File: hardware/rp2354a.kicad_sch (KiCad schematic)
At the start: 25 parts, among them J5 SM03B-SRSS-TB_LF__SN_, U1 RP2354A, Y1 ABM8-272-T3

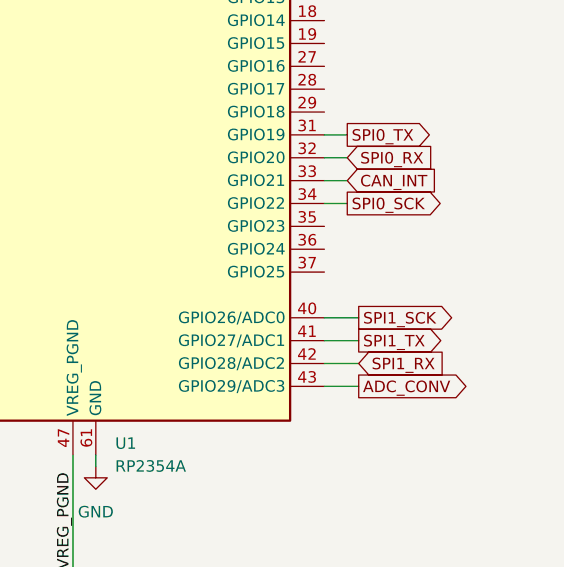
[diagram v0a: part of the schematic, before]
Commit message: Further iso bridge development
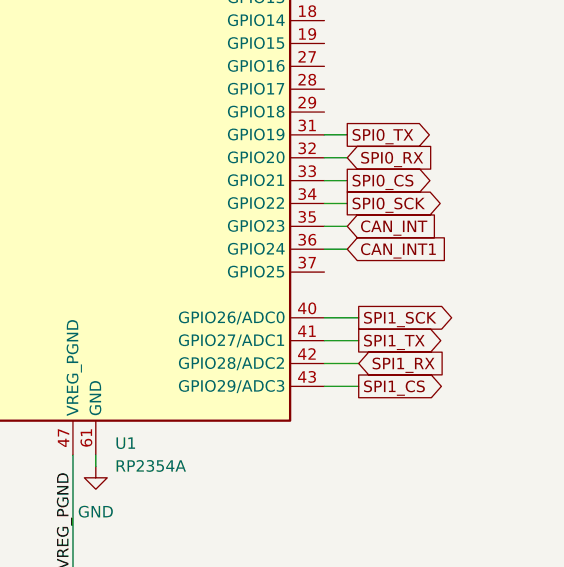
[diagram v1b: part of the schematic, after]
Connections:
- net CAN_INT: now also U1.35 (GPIO23); no longer U1.33 (GPIO21)
- net CAN_INT1: now reaches U1.36 (GPIO24)
- net ADC_CONV renamed SPI1_CS
- new net SPI0_CS: U1.33 (GPIO21)
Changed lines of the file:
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@@
+	(wire
+		(pts
+			(xy 175.26 88.9) (xy 187.96 88.9)
+		)
+		(stroke
+			(width 0)
+			(type default)
+		)
+	)
+	(wire
+		(pts
+			(xy 46.99 101.6) (xy 59.69 101.6)
+		)
+		(stroke
+			(width 0)
+			(type default)
+		)
+	)
+	(wire
+		(pts
+			(xy 166.37 29.21) (xy 154.94 29.21)
+		)
+		(stroke
+			(width 0)
+			(type default)
+		)
+	)
+	(wire
+		(pts
+			(xy 86.36 53.34) (xy 100.33 53.34)
+		)
+		(stroke
+			(width 0)
+			(type default)
+		)
+	)
+	(wire
+		(pts
+			(xy 91.44 127) (xy 46.99 127)
+		)
+		(stroke
+			(width 0)
+			(type default)
+		)
+	)
+	(wire
+		(pts
+			(xy 123.19 167.64) (xy 121.92 167.64)
+		)
+		(stroke
+			(width 0)
+			(type default)
+		)
+	)
+	(wire
+		(pts
+			(xy 203.2 46.99) (xy 208.28 46.99)
+		)
+		(stroke
+			(width 0)
+			(type default)
+		)
+	)
+	(wire
+		(pts
+			(xy 44.45 53.34) (xy 44.45 43.18)
+		)
+		(stroke
+			(width 0)
+			(type default)
+		)
+	)
+	(wire
+		(pts
+			(xy 39.37 53.34) (xy 44.45 53.34)
+		)
+		(stroke
+			(width 0)
+			(type default)
+		)
+	)
+	(wire
+		(pts
+			(xy 143.51 29.21) (xy 132.08 29.21)
+		)
+		(stroke
+			(width 0)
+			(type default)
+		)
+	)
+	(wire
+		(pts
+			(xy 91.44 43.18) (xy 85.09 43.18)
+		)
+		(stroke
+			(width 0)
+			(type default)
+		)
+	)
+	(wire
+		(pts
+			(xy 120.65 30.48) (xy 120.65 29.21)
+		)
+		(stroke
+			(width 0)
+			(type default)
+		)
+	)
+	(wire
+		(pts
+			(xy 88.9 88.9) (xy 78.74 88.9)
+		)
+		(stroke
+			(width 0)
+			(type default)
+		)
+	)
+	(wire
+		(pts
+			(xy 231.14 33.02) (xy 242.57 33.02)
+		)
+		(stroke
+			(width 0)
+			(type default)
+		)
+	)
+	(wire
+		(pts
+			(xy 154.94 39.37) (xy 166.37 39.37)
+		)
+		(stroke
+			(width 0)
+			(type default)
+		)
+	)
+	(wire
+		(pts
+			(xy 242.57 43.18) (xy 254 43.18)
+		)
+		(stroke
+			(width 0)
+			(type default)
+		)
+	)
 	(wire
 		(pts
@@
 	(wire
 		(pts
-			(xy 175.26 88.9) (xy 187.96 88.9)
-		)
-		(stroke
-			(width 0)
-			(type default)
-		)
-	)
-	(wire
-		(pts
-			(xy 46.99 101.6) (xy 59.69 101.6)
-		)
-		(stroke
-			(width 0)
-			(type default)
-		)
-	)
-	(wire
-		(pts
-			(xy 166.37 29.21) (xy 154.94 29.21)
-		)
-		(stroke
-			(width 0)
-			(type default)
-		)
-	)
-	(wire
-		(pts
-			(xy 86.36 53.34) (xy 100.33 53.34)
-		)
-		(stroke
-			(width 0)
-			(type default)
-		)
-	)
-	(wire
-		(pts
-			(xy 91.44 127) (xy 46.99 127)
-		)
-		(stroke
-			(width 0)
-			(type default)
-		)
-	)
-	(wire
-		(pts
-			(xy 123.19 167.64) (xy 121.92 167.64)
-		)
-		(stroke
-			(width 0)
-			(type default)
-		)
-	)
-	(wire
-		(pts
-			(xy 203.2 46.99) (xy 208.28 46.99)
-		)
-		(stroke
-			(width 0)
-			(type default)
-		)
-	)
-	(wire
-		(pts
-			(xy 44.45 53.34) (xy 44.45 43.18)
-		)
-		(stroke
-			(width 0)
-			(type default)
-		)
-	)
-	(wire
-		(pts
-			(xy 39.37 53.34) (xy 44.45 53.34)
-		)
-		(stroke
-			(width 0)
-			(type default)
-		)
-	)
-	(wire
-		(pts
-			(xy 143.51 29.21) (xy 132.08 29.21)
-		)
-		(stroke
-			(width 0)
-			(type default)
-		)
-	)
-	(wire
-		(pts
-			(xy 91.44 43.18) (xy 85.09 43.18)
-		)
-		(stroke
-			(width 0)
-			(type default)
-		)
-	)
-	(wire
-		(pts
-			(xy 120.65 30.48) (xy 120.65 29.21)
-		)
-		(stroke
-			(width 0)
-			(type default)
-		)
-	)
-	(wire
-		(pts
-			(xy 88.9 88.9) (xy 78.74 88.9)
-		)
-		(stroke
-			(width 0)
-			(type default)
-		)
-	)
-	(wire
-		(pts
-			(xy 231.14 33.02) (xy 242.57 33.02)
-		)
-		(stroke
-			(width 0)
-			(type default)
-		)
-	)
-	(wire
-		(pts
-			(xy 154.94 39.37) (xy 166.37 39.37)
-		)
-		(stroke
-			(width 0)
-			(type default)
-		)
-	)
-	(wire
-		(pts
-			(xy 242.57 43.18) (xy 254 43.18)
-		)
-		(stroke
-			(width 0)
-			(type default)
-		)
-	)
-	(wire
-		(pts
 			(xy 24.13 44.45) (xy 29.21 44.45)
 		)
@@
 	(wire
 		(pts
+			(xy 238.76 124.46) (xy 241.3 124.46)
+		)
+		(stroke
+			(width 0)
+			(type default)
+		)
+	)
+	(wire
+		(pts
 			(xy 166.37 30.48) (xy 166.37 29.21)
 		)
@@
 		(pts
 			(xy 220.98 43.18) (xy 220.98 55.88)
+		)
+		(stroke
+			(width 0)
+			(type default)
+		)
+	)
+	(wire
+		(pts
+			(xy 238.76 121.92) (xy 241.3 121.92)
 		)
 		(stroke
@@
 		)
 	)
+	(global_label "CAN_INT1"
+		(shape input)
+		(at 241.3 124.46 0)
+		(fields_autoplaced yes)
+		(effects
+			(font
+				(size 1.27 1.27)
+			)
+			(justify left)
+		)
+		(property "Intersheetrefs" "${INTERSHEET_REFS}"
+			(at 253.0543 124.46 0)
+			(hide yes)
+			(show_name no)
+			(do_not_autoplace no)
+			(effects
+				(font
+					(size 1.27 1.27)
+				)
+				(justify left)
+			)
+		)
+	)
 	(global_label "USB_D+"
 		(shape input)
@@
 	(global_label "CAN_INT"
 		(shape input)
+		(at 241.3 121.92 0)
+		(fields_autoplaced yes)
+		(effects
+			(font
+				(size 1.27 1.27)
+			)
+			(justify left)
+		)
+		(property "Intersheetrefs" "${INTERSHEET_REFS}"
+			(at 251.8448 121.92 0)
+			(hide yes)
+			(show_name no)
+			(do_not_autoplace no)
+			(effects
+				(font
+					(size 1.27 1.27)
+				)
+				(justify left)
+			)
+		)
+	)
+	(global_label "SPI0_CS"
+		(shape output)
 		(at 241.3 116.84 0)
 		(fields_autoplaced yes)
@@
 		)
 		(property "Intersheetrefs" "${INTERSHEET_REFS}"
-			(at 251.8448 116.84 0)
+			(at 252.0261 116.84 0)
 			(hide yes)
 			(show_name no)
@@
 		)
 	)
-	(global_label "ADC_CONV"
+	(global_label "SPI1_CS"
 		(shape output)
 		(at 242.57 139.7 0)
@@
 		)
 		(property "Intersheetrefs" "${INTERSHEET_REFS}"
-			(at 255.171 139.7 0)
+			(at 253.2961 139.7 0)
 			(hide yes)
 			(show_name no)
